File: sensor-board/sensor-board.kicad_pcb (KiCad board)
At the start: 2 copper layers, 45 x 24 mm, 18 parts, among them J1 Batt, J2 I2C, Q1 DMG3415U-7, U1 MCP73831-3-OT, U2 Arduino-nano-BLE-33, U3 MCP1700T-3102, U4 SGP40-D-R4

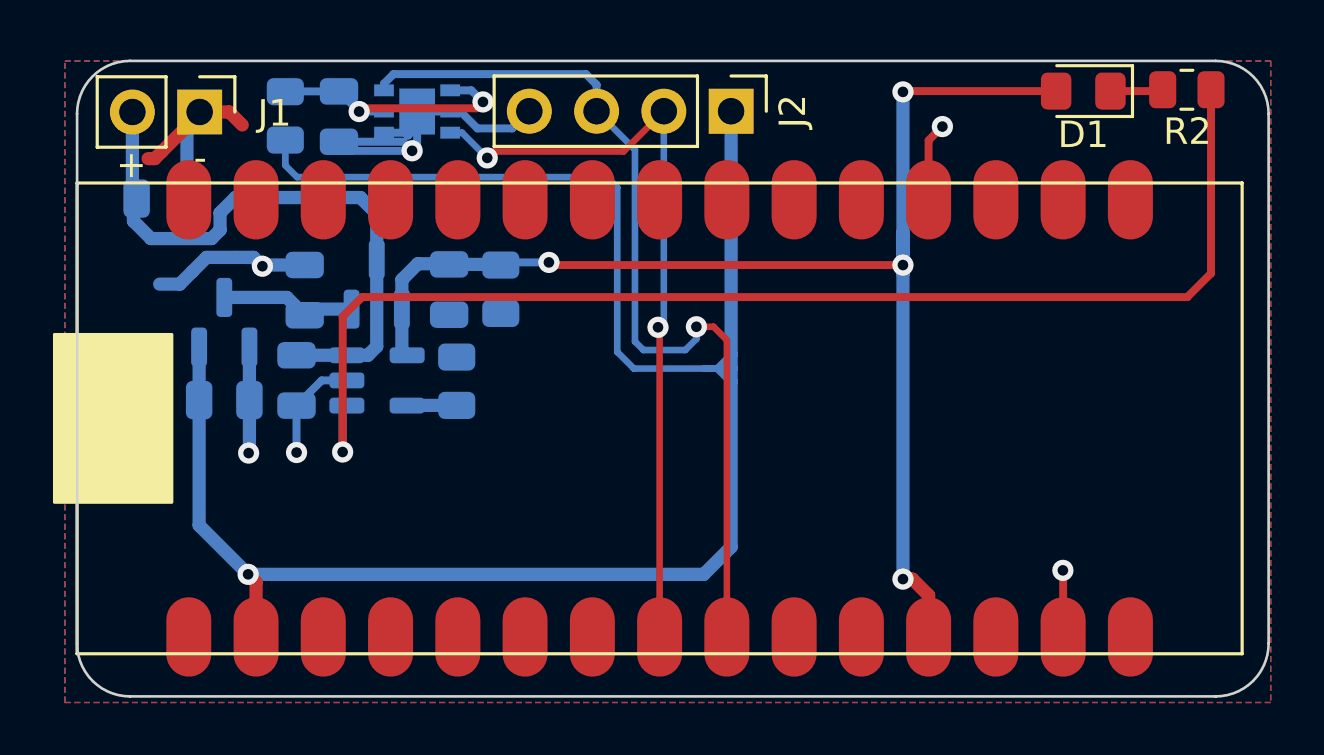
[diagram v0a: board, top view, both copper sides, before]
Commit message: update sensor board v1.0
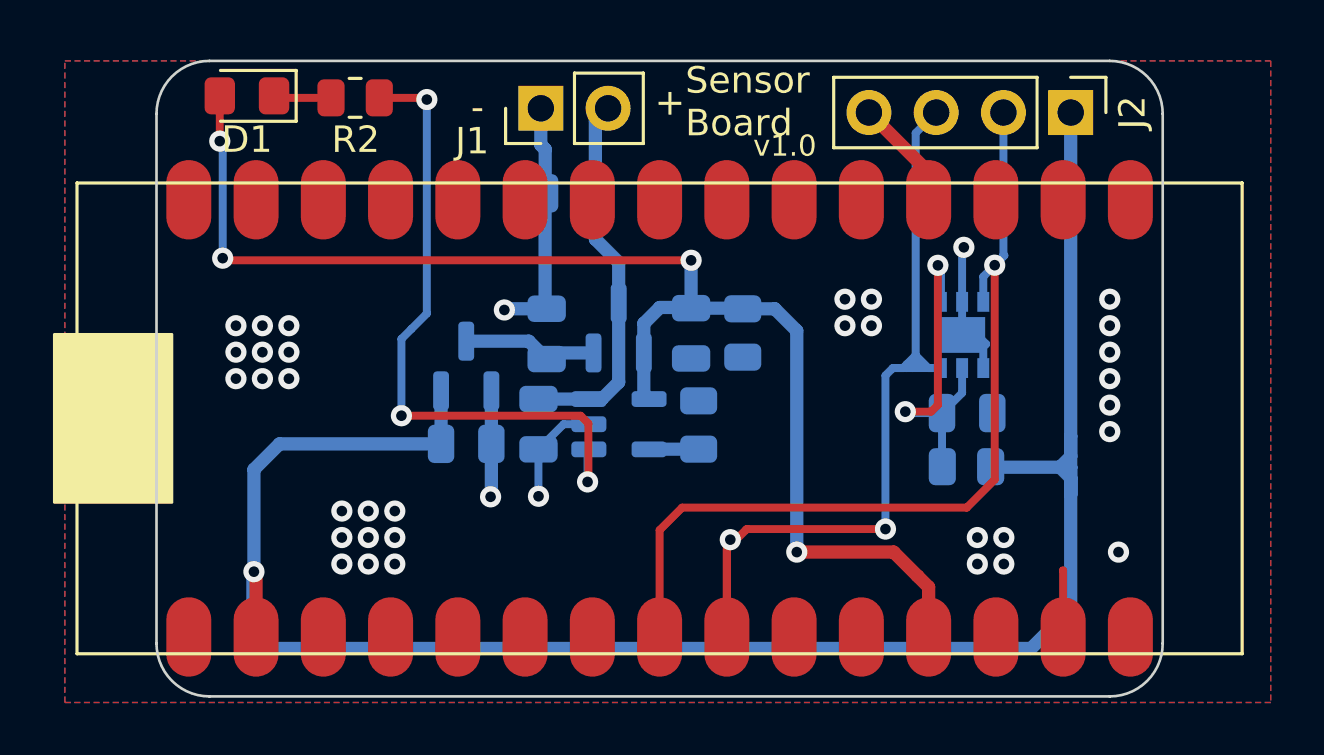
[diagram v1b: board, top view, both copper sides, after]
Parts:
- moved D1 31.6 mm to (126.4, 57.3)
- moved R2 31.4 mm to (130.5, 57.4)
- moved R4 28.9 mm to (153.6, 71.3), turned to 0 degrees
- moved C6 26.2 mm to (153.6, 69.3), turned to 0 degrees
- moved U4 22.2 mm to (153.4, 66.3), turned to -90 degrees
- moved C4 15.4 mm to (138.6, 61.0), turned to 180 degrees
- moved J1 12.9 mm to (137.5, 57.8), turned to 90 degrees
- moved J2 12.8 mm to (157.5, 58.0)
- moved C1 9.29 mm to (137.4, 69.7)
- moved C2 9.29 mm to (137.7, 66.3)
- moved C5 9.29 mm to (134.7, 70.5)
- moved Q1 9.29 mm to (140.5, 66.1)
- moved R1 9.29 mm to (143.5, 69.8)
- moved R3 9.29 mm to (145.1, 66.3)
- moved U1 9.29 mm to (140.5, 69.7)
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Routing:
- net Net-(R2-Pad1): track 47.3 -> 25.0 mm, vias 1 -> 3
- net GND: track 41.8 -> 29.5 mm, vias 6 -> 37
- net +BATT: track 23.2 -> 14.2 mm
- net VBUS: track 57.3 -> 50.8 mm
- net /SDA: track 29.2 -> 33.1 mm, vias 2 -> 1
- net Net-(C6-Pad1): track 10.3 -> 13.5 mm
- net /SCL: track 34.6 -> 33.7 mm, vias 1 -> 2
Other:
- board size 45 x 24 mm -> 38 x 24 mm
- board text added: "Sensor Board"
- board text added: "v1.0"
